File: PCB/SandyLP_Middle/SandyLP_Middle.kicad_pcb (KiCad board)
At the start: 2 copper layers, 113.1 x 56.3 mm, 110 parts

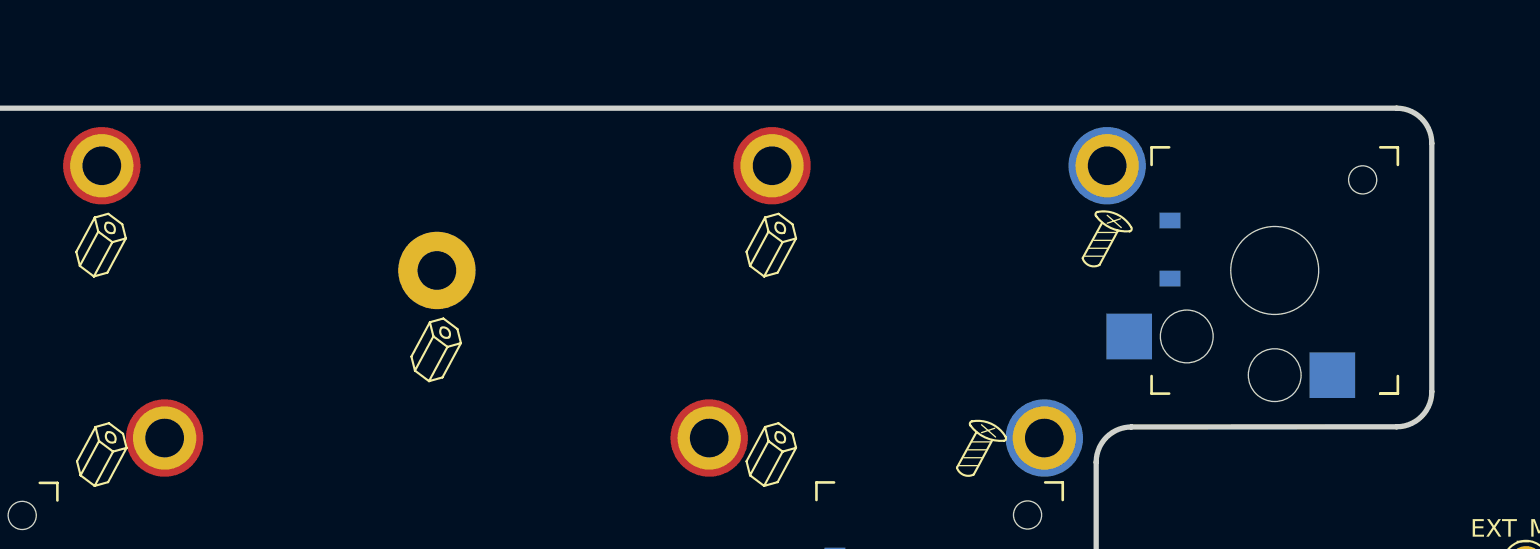
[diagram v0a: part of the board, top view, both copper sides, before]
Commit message: 不要なものを整理。
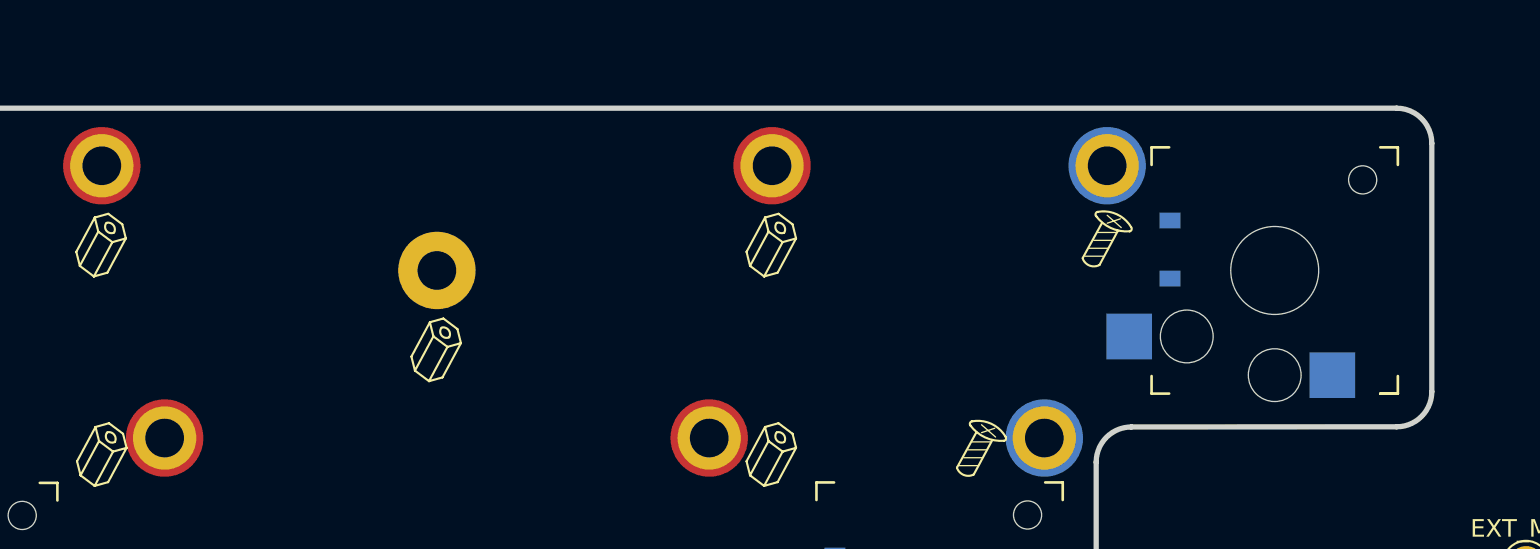
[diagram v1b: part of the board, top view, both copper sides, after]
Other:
- board text removed: "to Base"
- board text removed: "to Top"
